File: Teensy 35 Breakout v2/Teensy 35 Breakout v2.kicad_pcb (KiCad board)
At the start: 2 copper layers, 99.1 x 106.7 mm, 41 parts, among them P1 CONN_01X13, P10 CONN_01X13, P10a1 CONN_01X10, P11 CONN_01X03, P12 CONN_01X04, P13 CONN_02X04, P14 CONN_02X03, P15 CONN_02X05, P16 CONN_01X03, P17 CONN_01X01, P18 CONN_01X02, P19 CONN_01X08, P1a1 CONN_01X09, P2 CONN_01X13, P20 CONN_01X05, P21 CONN_01X05, P22 CONN_01X04, P23 CONN_01X04, P24 CONN_01X05, P25 CONN_01X10, P26 CONN_01X10, P27 CONN_01X10, P28 CONN_01X10, P2a1 CONN_01X09, P2a2 CONN_01X03, P2a3 CONN_01X03, P3 CONN_01X03, P4 CONN_01X24, P5 CONN_01X24, P6 CONN_01X03, P7 CONN_01X24, P8 CONN_01X24, P9 CONN_01X13, P9a1 CONN_01X09, SW1 SW_PUSH_SMALL_H, SW2 SW_PUSH_SMALL_H

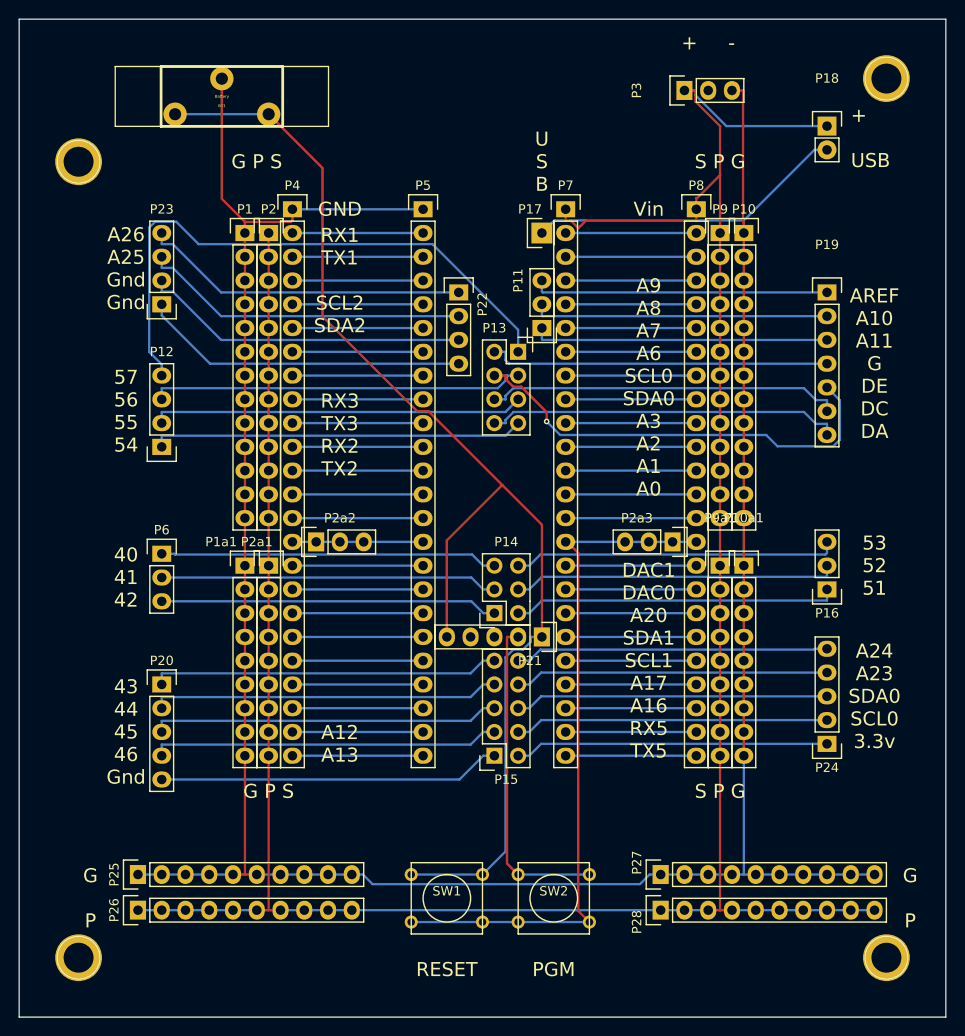
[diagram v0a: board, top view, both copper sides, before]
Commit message: Final updates and corrections
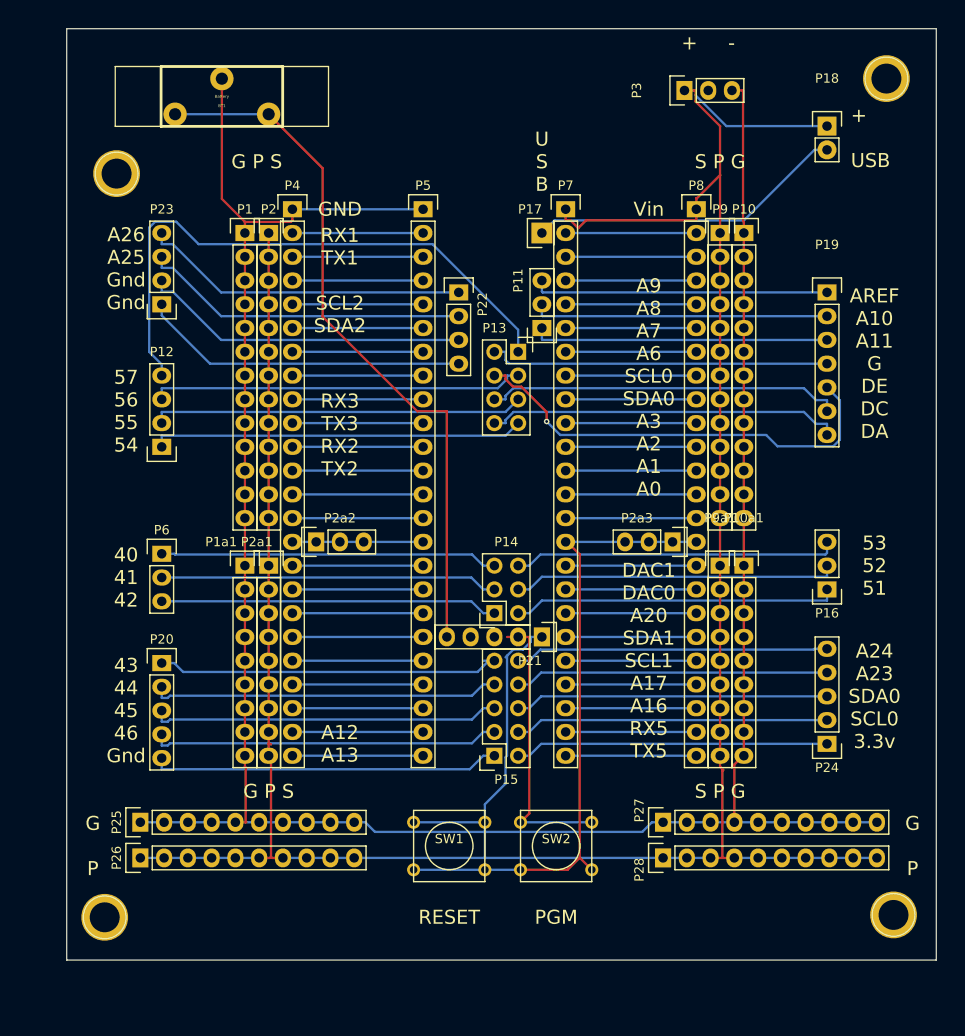
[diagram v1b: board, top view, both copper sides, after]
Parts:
- moved P27 5.59 mm to (129.8, 116.3)
- moved P28 5.59 mm to (129.8, 120.1)
- moved P25 5.59 mm to (73.9, 116.3)
- moved P26 5.59 mm to (73.9, 120.1)
- moved SW1 5.59 mm to (106.9, 118.9)
- moved SW2 5.59 mm to (118.4, 118.9)
- moved REF3 5.14 mm to (70.1, 126.5)
- moved RE4 4.64 mm to (154.4, 126.2)
- moved REF2 4.26 mm to (71.4, 47.0)
- moved P20 2.29 mm to (76.2, 99.3)
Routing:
- net Net-(P21-Pad1): track 49.0 -> 35.3 mm
- net Net-(P18-Pad1): track 278.8 -> 267.1 mm
- net Net-(BT1-Pad1): track 85.4 -> 75.6 mm
- net Net-(BT1-Pad2): track 271.0 -> 261.7 mm
- net Net-(P2a3-Pad1): track 74.8 -> 68.6 mm
- net Net-(P21-Pad2): track 34.7 -> 30.2 mm
- net Net-(P7-Pad1): track 1.19 -> 2.88 mm
- net Net-(P15-Pad1): track 36.6 -> 37.3 mm
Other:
- board size 99.1 x 106.7 mm -> 93 x 99.6 mm

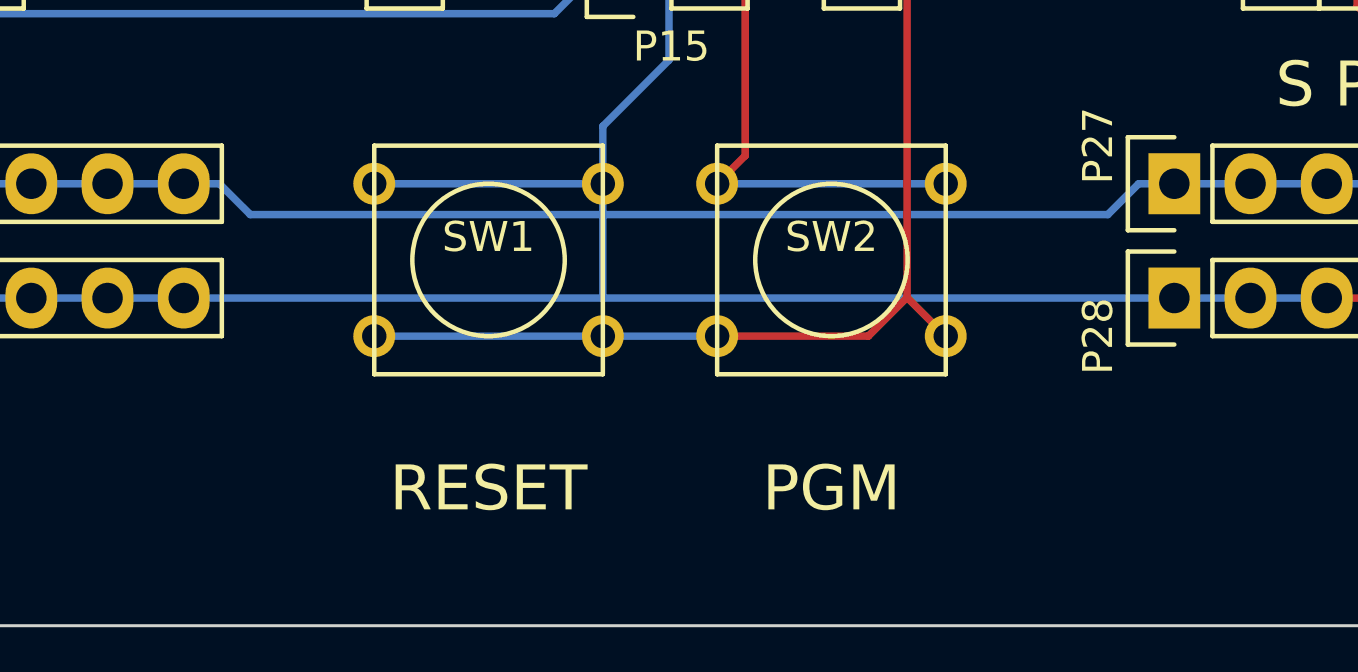
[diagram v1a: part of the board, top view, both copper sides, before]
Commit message: Correcyrf some connections
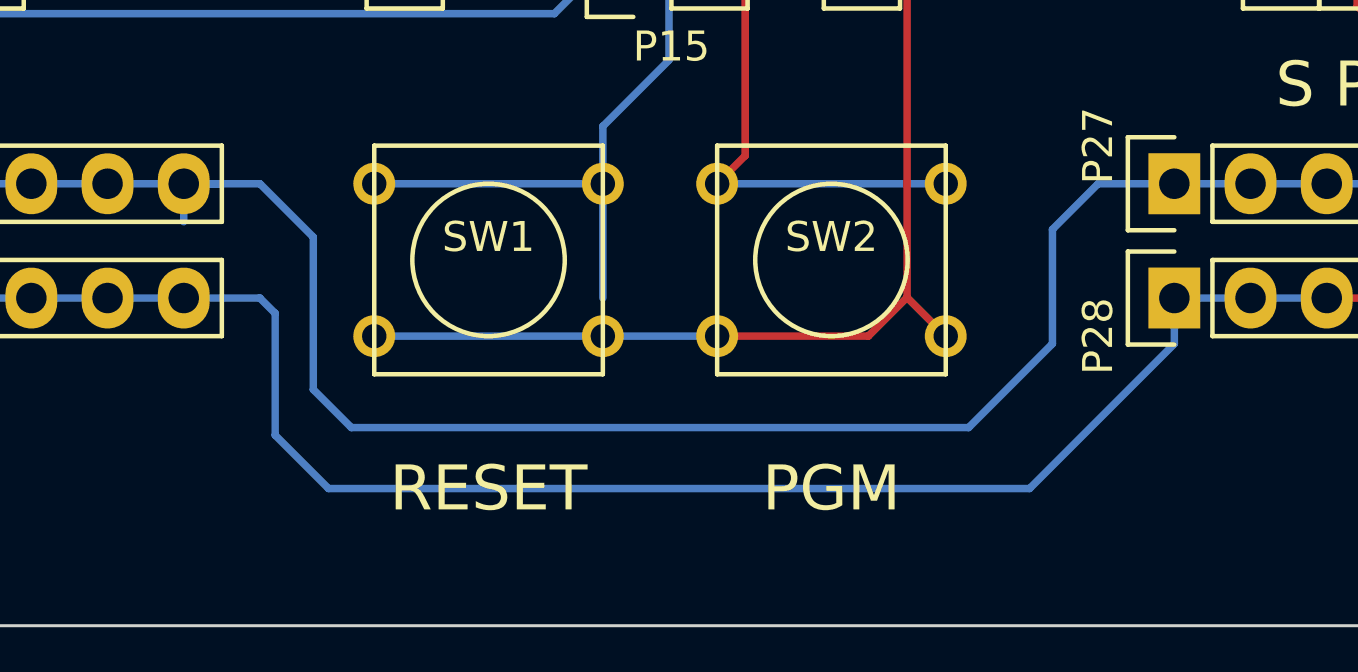
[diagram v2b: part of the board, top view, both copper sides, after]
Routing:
- net Net-(BT1-Pad2): track 261.7 -> 275.3 mm
- net Net-(P18-Pad1): track 267.1 -> 276.8 mm
- net Net-(P7-Pad1): track 2.88 -> 1.71 mm
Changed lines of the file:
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@@
     (thickness 1.6)
     (drawings 29)
-    (tracks 414)
+    (tracks 426)
     (zones 0)
     (modules 41)
@@
   (segment (start 93.3926 62.2691) (end 93.3926 46.4026) (width 0.25) (layer F.Cu) (net 1))
   (segment (start 103.514 72.39) (end 93.3926 62.2691) (width 0.25) (layer F.Cu) (net 1))
+  (segment (start 96.774 116.332) (end 99.314 116.332) (width 0.25) (layer B.Cu) (net 2))
+  (segment (start 99.314 116.332) (end 101.092 118.11) (width 0.25) (layer B.Cu) (net 2))
+  (segment (start 101.092 118.11) (end 101.092 123.19) (width 0.25) (layer B.Cu) (net 2))
+  (segment (start 101.092 123.19) (end 102.362 124.46) (width 0.25) (layer B.Cu) (net 2))
+  (segment (start 102.362 124.46) (end 122.936 124.46) (width 0.25) (layer B.Cu) (net 2))
+  (segment (start 122.936 124.46) (end 125.73 121.666) (width 0.25) (layer B.Cu) (net 2))
+  (segment (start 125.73 121.666) (end 125.73 117.856) (width 0.25) (layer B.Cu) (net 2))
+  (segment (start 125.73 117.856) (end 127.254 116.332) (width 0.25) (layer B.Cu) (net 2))
+  (segment (start 127.254 116.332) (end 129.794 116.332) (width 0.25) (layer B.Cu) (net 2))
+  (segment (start 96.774 116.332) (end 96.774 117.598) (width 0.25) (layer B.Cu) (net 2))
   (segment (start 138.349 38.1) (end 137.16 38.1) (width 0.25) (layer F.Cu) (net 2))
   (segment (start 138.349 52.07) (end 138.349 38.1) (width 0.25) (layer F.Cu) (net 2))
@@
   (segment (start 85.09 109.22) (end 85.09 106.68) (width 0.25) (layer F.Cu) (net 2))
   (segment (start 132.334 116.332) (end 129.794 116.332) (width 0.25) (layer B.Cu) (net 2))
-  (segment (start 128.605 116.332) (end 129.794 116.332) (width 0.25) (layer B.Cu) (net 2))
-  (segment (start 127.577 117.36) (end 128.605 116.332) (width 0.25) (layer B.Cu) (net 2))
-  (segment (start 98.9914 117.36) (end 127.577 117.36) (width 0.25) (layer B.Cu) (net 2))
-  (segment (start 97.9629 116.332) (end 98.9914 117.36) (width 0.25) (layer B.Cu) (net 2))
   (segment (start 96.774 116.332) (end 97.9629 116.332) (width 0.25) (layer B.Cu) (net 2))
   (segment (start 96.774 116.332) (end 94.234 116.332) (width 0.25) (layer B.Cu) (net 2))
@@
   (segment (start 85.09 110.409) (end 85.1765 110.4956) (width 0.25) (layer F.Cu) (net 2))
   (segment (start 85.09 109.22) (end 85.09 110.409) (width 0.25) (layer F.Cu) (net 2))
+  (segment (start 96.774 120.142) (end 99.314 120.142) (width 0.25) (layer B.Cu) (net 3))
+  (segment (start 99.314 120.142) (end 99.822 120.65) (width 0.25) (layer B.Cu) (net 3))
+  (segment (start 99.822 120.65) (end 99.822 124.714) (width 0.25) (layer B.Cu) (net 3))
+  (segment (start 99.822 124.714) (end 101.6 126.492) (width 0.25) (layer B.Cu) (net 3))
+  (segment (start 101.6 126.492) (end 124.968 126.492) (width 0.25) (layer B.Cu) (net 3))
+  (segment (start 124.968 126.492) (end 129.794 121.666) (width 0.25) (layer B.Cu) (net 3))
+  (segment (start 129.794 121.666) (end 129.794 120.142) (width 0.25) (layer B.Cu) (net 3))
   (segment (start 136.559 41.91) (end 147.32 41.91) (width 0.25) (layer B.Cu) (net 3))
   (segment (start 133.269 38.6201) (end 136.559 41.91) (width 0.25) (layer B.Cu) (net 3))
@@
   (segment (start 135.89 81.28) (end 135.89 78.74) (width 0.25) (layer F.Cu) (net 3))
   (segment (start 135.89 109.22) (end 135.89 106.68) (width 0.25) (layer F.Cu) (net 3))
-  (segment (start 129.794 120.142) (end 96.774 120.142) (width 0.25) (layer B.Cu) (net 3))
   (segment (start 87.803 107.95) (end 87.884 108.031) (width 0.25) (layer F.Cu) (net 3))
   (segment (start 87.63 107.95) (end 87.803 107.95) (width 0.25) (layer F.Cu) (net 3))
@@
   (segment (start 136.144 120.142) (end 136.144 110.825) (width 0.25) (layer F.Cu) (net 3))
   (segment (start 121.562 51.9889) (end 120.731 52.8197) (width 0.25) (layer F.Cu) (net 3))
+  (segment (start 120.731 52.8197) (end 119.9 51.9889) (width 0.25) (layer F.Cu) (net 3))
   (segment (start 90.17 86.36) (end 92.71 86.36) (width 0.25) (layer B.Cu) (net 4))
   (segment (start 104.14 86.36) (end 97.79 86.36) (width 0.25) (layer B.Cu) (net 4))
@@
   (segment (start 119.38 51.9889) (end 119.38 50.8) (width 0.25) (layer F.Cu) (net 87))
   (segment (start 119.9 51.9889) (end 119.38 51.9889) (width 0.25) (layer F.Cu) (net 87))
-  (segment (start 120.731 52.8197) (end 119.9 51.9889) (width 0.25) (layer F.Cu) (net 87))
 )
